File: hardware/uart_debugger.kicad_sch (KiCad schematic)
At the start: 3 parts, among them Q3 JSM2302, U3 CH340E UART Module

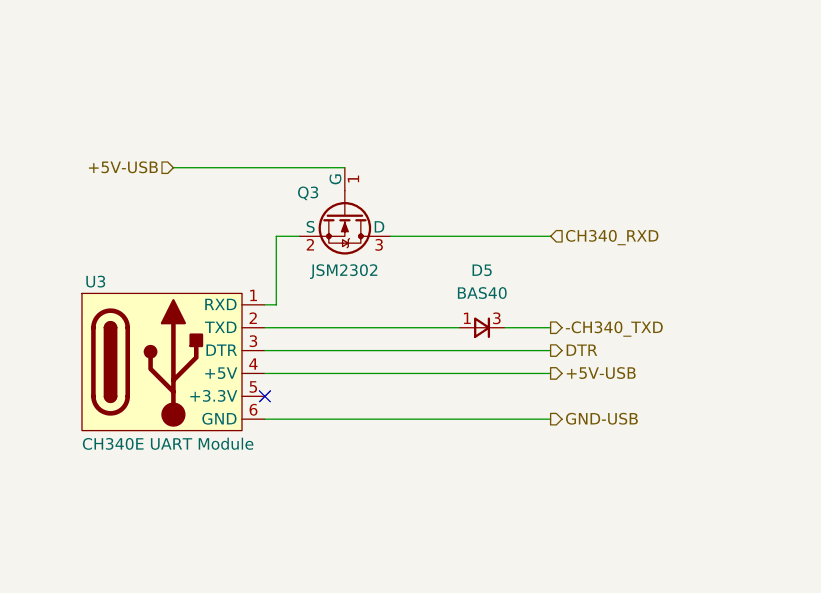
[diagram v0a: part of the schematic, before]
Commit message: Electric Rules Check completed.
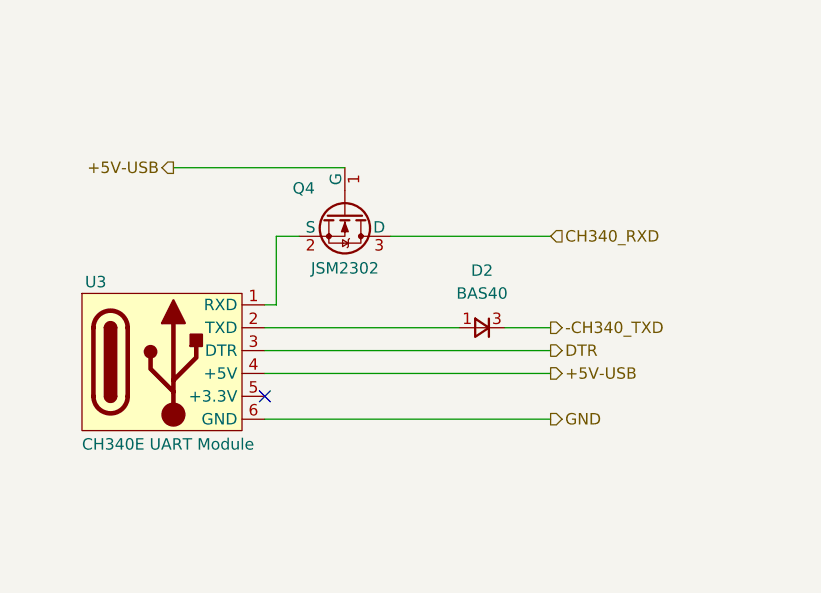
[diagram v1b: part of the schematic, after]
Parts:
- removed D5: BAS40, Package_TO_SOT_SMD:SOT-23, symbol Device:D_Small
- removed Q3: JSM2302, Package_TO_SOT_SMD:SOT-23, symbol Simulation_SPICE:NMOS
- added D2: BAS40, Package_TO_SOT_SMD:SOT-23, symbol kitchen_timer-symbols_lib:BAS40_diode
- added Q4: JSM2302, Package_TO_SOT_SMD:SOT-23, symbol kitchen_timer-symbols_lib:JSM2302
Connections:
- net +5V-USB: now also Q4.1 (G)
- net CH340_RXD: now also Q4.3 (D)
- net ­CH340_TXD: now also D2.3 (K)
- net at U3.1 (RXD): now also Q4.2 (S)
- net at U3.2 (TXD): now also D2.1 (A)
- net GND-USB renamed GND
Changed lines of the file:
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@@
 	)
 	(hierarchical_label "+5V-USB"
-		(shape input)
+		(shape output)
 		(at 125.73 82.55 180)
 		(effects
@@
 		)
 	)
-	(hierarchical_label "GND-USB"
+	(hierarchical_label "GND"
 		(shape output)
 		(at 167.64 110.49 0)
@@
 	)
 	(symbol
-		(lib_id "Simulation_SPICE:NMOS")
+		(lib_id "kitchen_timer-symbols_lib:BAS40_diode")
+		(at 160.02 100.33 180)
+		(unit 1)
+		(exclude_from_sim no)
+		(in_bom yes)
+		(on_board yes)
+		(dnp no)
+		(fields_autoplaced yes)
+		(property "Reference" "D2"
+			(at 160.02 93.98 0)
+			(effects
+				(font
+					(size 1.27 1.27)
+				)
+			)
+		)
+		(property "Value" "BAS40"
+			(at 160.02 96.52 0)
+			(effects
+				(font
+					(size 1.27 1.27)
+				)
+			)
+		)
+		(property "Footprint" "Package_TO_SOT_SMD:SOT-23"
+			(at 138.938 100.076 90)
+			(effects
+				(font
+					(size 1.27 1.27)
+				)
+				(hide yes)
+			)
+		)
+		(property "Datasheet" "https://jlcpcb.com/api/file/downloadByFileSystemAccessId/8590224761860497408"
+			(at 142.748 101.092 90)
+			(effects
+				(font
+					(size 1.27 1.27)
+				)
+				(hide yes)
+			)
+		)
+		(property "Description" "40V Independent Type 200mA 1V@40mA SOT-23 Schottky Diodes ROHS"
+			(at 158.75 118.872 0)
+			(effects
+				(font
+					(size 1.27 1.27)
+				)
+				(hide yes)
+			)
+		)
+		(property "Sim.Pins" "1=K 2=A"
+			(at 148.844 110.998 0)
+			(effects
+				(font
+					(size 1.27 1.27)
+				)
+				(hide yes)
+			)
+		)
+		(property "Supplier Link" "https://jlcpcb.com/partdetail/78417-BAS40/C77289"
+			(at 156.21 121.412 0)
+			(effects
+				(font
+					(size 1.27 1.27)
+				)
+				(hide yes)
+			)
+		)
+		(property "Package" "SOT-23"
+			(at 158.496 115.316 0)
+			(effects
+				(font
+					(size 1.27 1.27)
+				)
+				(hide yes)
+			)
+		)
+		(property "Supplier Name" "JLCPCB"
+			(at 160.02 100.33 0)
+			(effects
+				(font
+					(size 1.27 1.27)
+				)
+				(hide yes)
+			)
+		)
+		(property "Manuf. Part #" "BAS40"
+			(at 160.02 100.33 0)
+			(effects
+				(font
+					(size 1.27 1.27)
+				)
+				(hide yes)
+			)
+		)
+		(property "Supplier Unit Price" "$0.0257"
+			(at 160.02 100.33 0)
+			(effects
+				(font
+					(size 1.27 1.27)
+				)
+				(hide yes)
+			)
+		)
+		(property "Part Num" "NA"
+			(at 160.02 100.33 0)
+			(effects
+				(font
+					(size 1.27 1.27)
+				)
+				(hide yes)
+			)
+		)
+		(property "Manuf. Name" "Jiangsu Changjing Electronics Technology Co., Ltd."
+			(at 160.02 100.33 0)
+			(effects
+				(font
+					(size 1.27 1.27)
+				)
+				(hide yes)
+			)
+		)
+		(property "Supplier Part #" " C77289"
+			(at 160.02 100.33 0)
+			(effects
+				(font
+					(size 1.27 1.27)
+				)
+				(hide yes)
+			)
+		)
+		(pin "3"
+		)
+		(pin "1"
+		)
+		(instances
+			(project ""
+				(path "/8963deea-96bc-4401-b671-98fbe9ed9c6a/f7e640d9-c0d9-4c44-8592-f18e152ed7d5"
+					(reference "D2")
+					(unit 1)
+				)
+			)
+		)
+	)
+	(symbol
+		(lib_id "kitchen_timer-symbols_lib:JSM2302")
 		(at 144.78 87.63 270)
 		(unit 1)
@@
 		(on_board yes)
 		(dnp no)
-		(property "Reference" "Q3"
-			(at 140.716 85.344 90)
+		(property "Reference" "Q4"
+			(at 140.208 84.836 90)
 			(effects
 				(font
@@
 		)
 		(property "Value" "JSM2302"
-			(at 144.78 93.98 90)
+			(at 144.78 93.726 90)
 			(effects
 				(font
@@
 			)
 		)
-		(property "Sim.Type" "VDMOS"
+		(property "Sim.Type" ""
 			(at 125.73 87.63 0)
 			(effects
@@
 			)
 		)
-		(property "Sim.Pins" "1=D 2=G 3=S"
+		(property "Sim.Pins" ""
 			(at 129.54 87.63 0)
 			(effects
@@
 			(project ""
 				(path "/8963deea-96bc-4401-b671-98fbe9ed9c6a/f7e640d9-c0d9-4c44-8592-f18e152ed7d5"
-					(reference "Q3")
+					(reference "Q4")
 					(unit 1)
 				)
-			)
-		)
-	)
-	(symbol
-		(lib_name "D_Small_1")
-		(lib_id "Device:D_Small")
-		(at 160.02 100.33 0)
-		(mirror y)
-		(unit 1)
-		(exclude_from_sim no)
-		(in_bom yes)
-		(on_board yes)
-		(dnp no)
-		(property "Reference" "D5"
-			(at 160.02 93.98 0)
-			(effects
-				(font
-					(size 1.27 1.27)
-				)
-			)
-		)
-		(property "Value" "BAS40"
-			(at 160.02 96.52 0)
-			(effects
-				(font
-					(size 1.27 1.27)
-				)
-			)
-		)
-		(property "Footprint" "Package_TO_SOT_SMD:SOT-23"
-			(at 138.938 100.584 90)
-			(effects
-				(font
-					(size 1.27 1.27)
-				)
-				(hide yes)
-			)
-		)
-		(property "Datasheet" "https://jlcpcb.com/api/file/downloadByFileSystemAccessId/8590224761860497408"
-			(at 142.748 99.568 90)
-			(effects
-				(font
-					(size 1.27 1.27)
-				)
-				(hide yes)
-			)
-		)
-		(property "Description" "40V Independent Type 200mA 1V@40mA SOT-23 Schottky Diodes ROHS"
-			(at 158.75 81.788 0)
-			(effects
-				(font
-					(size 1.27 1.27)
-				)
-				(hide yes)
-			)
-		)
-		(property "Sim.Pins" "1=K 2=A"
-			(at 148.844 89.662 0)
-			(effects
-				(font
-					(size 1.27 1.27)
-				)
-				(hide yes)
-			)
-		)
-		(property "Supplier Link" "https://jlcpcb.com/partdetail/78417-BAS40/C77289"
-			(at 156.21 79.248 0)
-			(effects
-				(font
-					(size 1.27 1.27)
-				)
-				(hide yes)
-			)
-		)
-		(property "Package" "SOT-23"
-			(at 158.496 85.344 0)
-			(effects
-				(font
-					(size 1.27 1.27)
-				)
-				(hide yes)
-			)
-		)
-		(property "Supplier Name" "JLCPCB"
-			(at 160.02 100.33 0)
-			(effects
-				(font
-					(size 1.27 1.27)
-				)
-				(hide yes)
-			)
-		)
-		(property "Manuf. Part #" "BAS40"
-			(at 160.02 100.33 0)
-			(effects
-				(font
-					(size 1.27 1.27)
-				)
-				(hide yes)
-			)
-		)
-		(property "Supplier Unit Price" "$0.0257"
-			(at 160.02 100.33 0)
-			(effects
-				(font
-					(size 1.27 1.27)
-				)
-				(hide yes)
-			)
-		)
-		(property "Part Num" "NA"
-			(at 160.02 100.33 0)
-			(effects
-				(font
-					(size 1.27 1.27)
-				)
-				(hide yes)
-			)
-		)
-		(property "Manuf. Name" "Jiangsu Changjing Electronics Technology Co., Ltd."
-			(at 160.02 100.33 0)
-			(effects
-				(font
-					(size 1.27 1.27)
-				)
-				(hide yes)
-			)
-		)
-		(property "Supplier Part #" " C77289"
-			(at 160.02 100.33 0)
-			(effects
-				(font
-					(size 1.27 1.27)
-				)
-				(hide yes)
-			)
-		)
-		(pin "3"
-		)
-		(pin "1"
-		)
-		(instances
-			(project "kitchen_timer-hardware"
-				(path "/8963deea-96bc-4401-b671-98fbe9ed9c6a/f7e640d9-c0d9-4c44-8592-f18e152ed7d5"
-					(reference "D5")
-					(unit 1)
-				)
